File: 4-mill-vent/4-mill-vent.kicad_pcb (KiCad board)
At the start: 2 copper layers, 76.2 x 47.6 mm, 78 parts, among them J1 Fan, J2 Buzzer, J3 Power, J4 ICSP, Q1 MMBT3904, Q2 MMBT3904, Q3 PZT3904, Q4 PZT3904, Q5 TSM480P06CP, Q6 MMBT3904, Q7 MMBT3904, SW1 Power_off, SW2 Power_On, SW3 Fan_Down, SW4 Fan_Up, U1 LM321, U2 ATmega328P-AU, U3 TPSM84212EAB, U4 LM1117-5.0, Y1 16.000MHZ

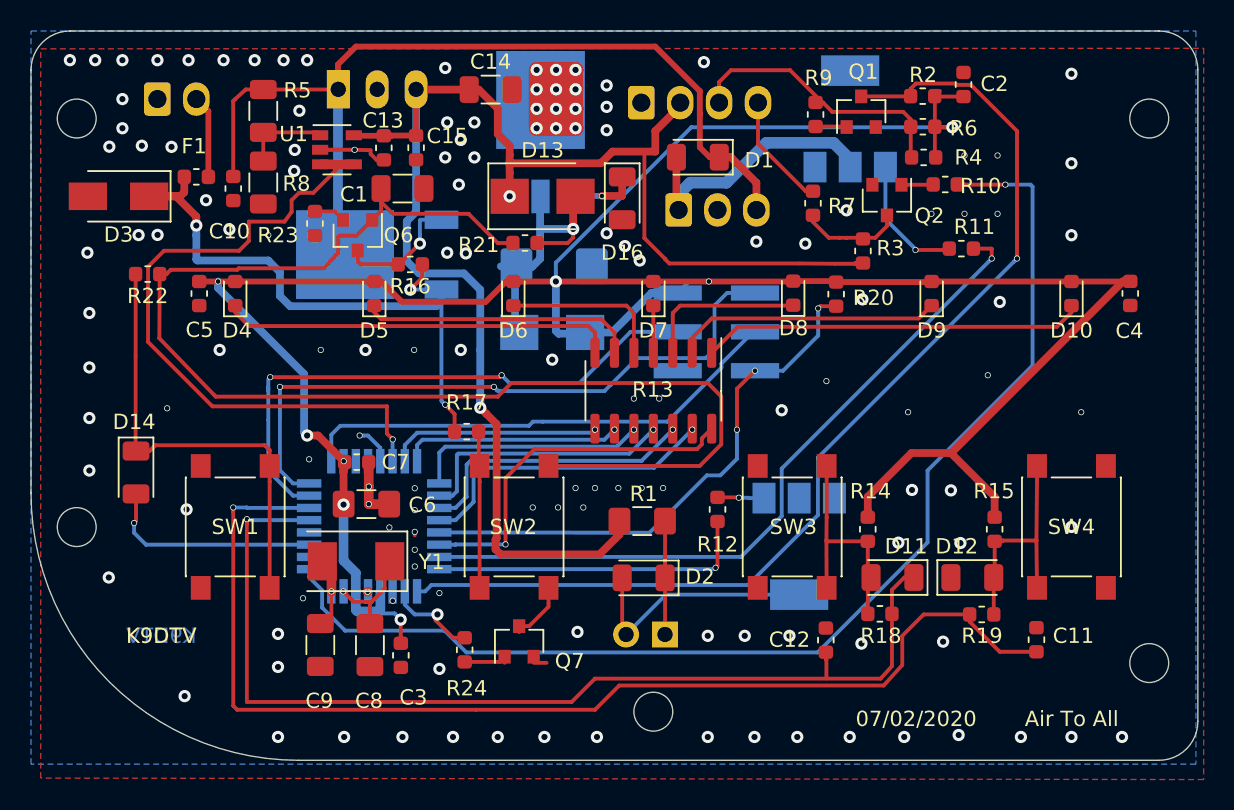
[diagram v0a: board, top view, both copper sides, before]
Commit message: more clean up
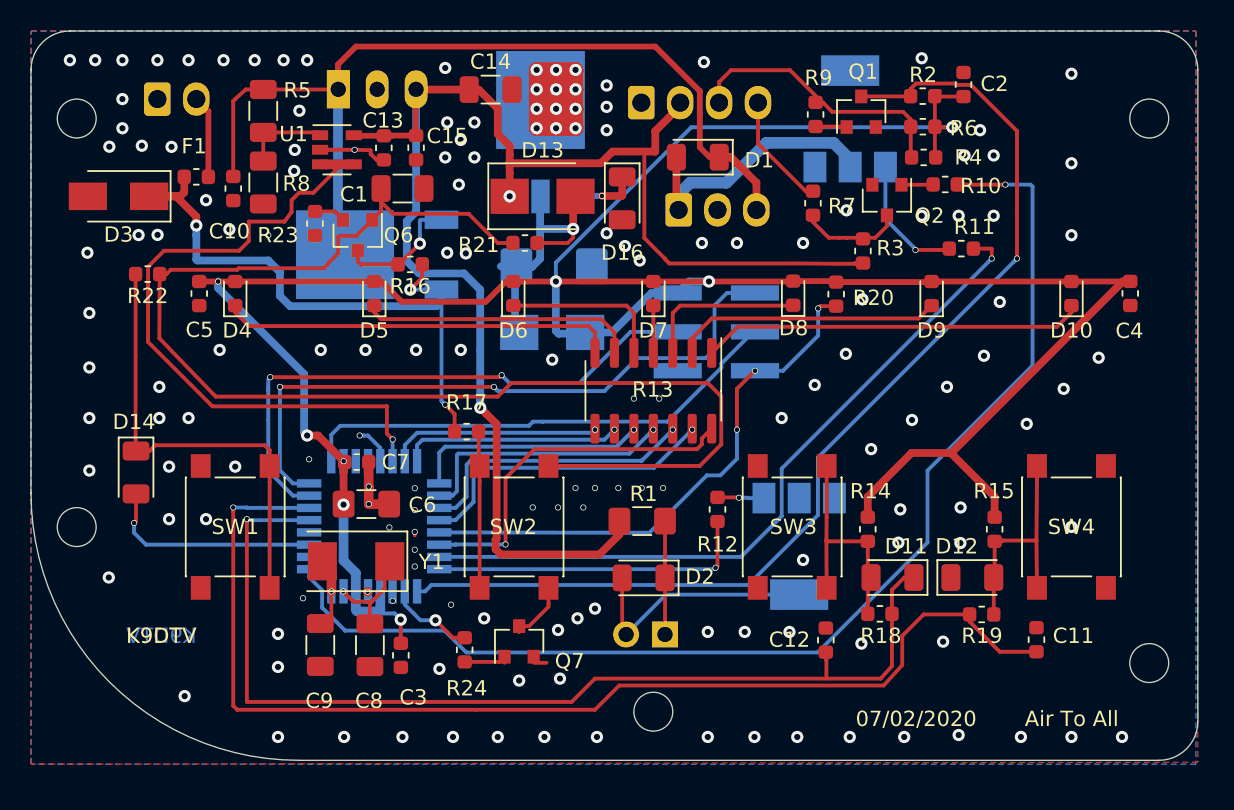
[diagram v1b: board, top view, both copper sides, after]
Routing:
- net GND: vias 126 -> 145
